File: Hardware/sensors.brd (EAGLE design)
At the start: 45.7 x 35.6 mm, 19 parts, among them IC1 74AC11D, IC2 REG1117

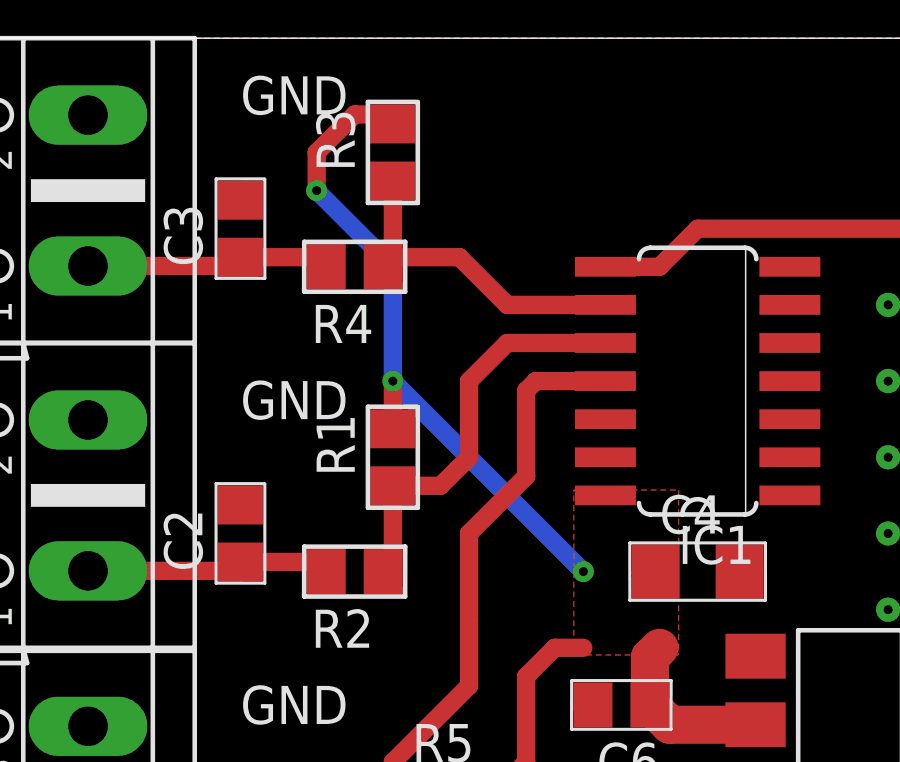
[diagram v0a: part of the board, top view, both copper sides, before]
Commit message: Fix some componenent manufacturer reference
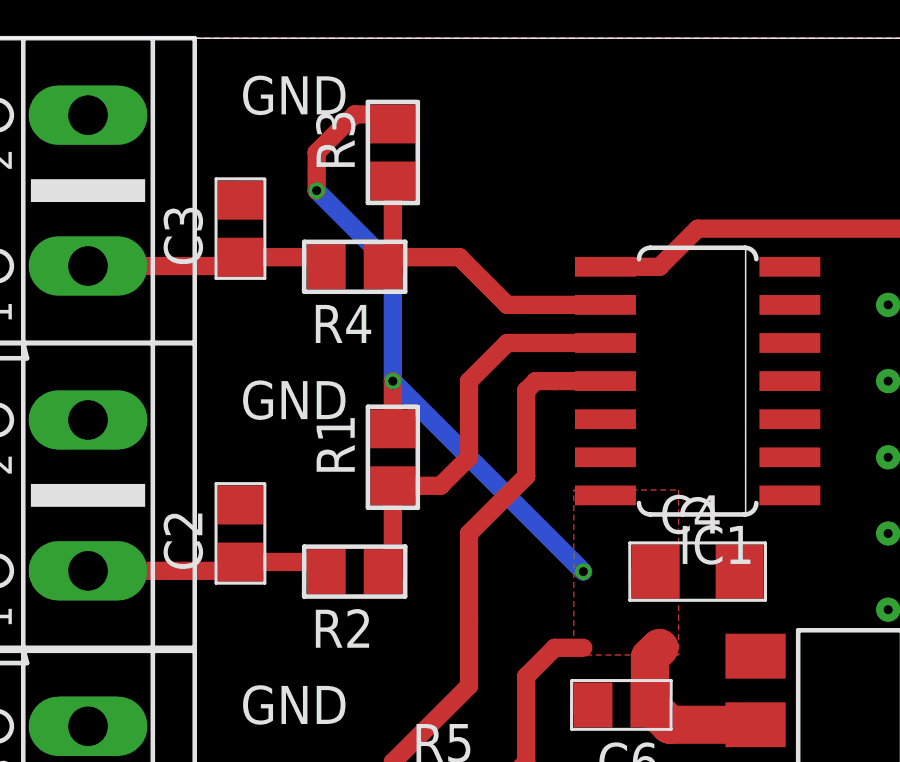
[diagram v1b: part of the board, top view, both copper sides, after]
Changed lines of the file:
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@@
 </class>
 </classes>
-<designrules name="default *">
-<description language="de">&lt;b&gt;EAGLE Design Rules&lt;/b&gt;
+<designrules name="jlcpcb2layer">
+<description language="en">&lt;b&gt;JLCPCB Design Rules by Jaap de Dood&lt;/b&gt;
 &lt;p&gt;
-Die Standard-Design-Rules sind so gewählt, dass sie für
-die meisten Anwendungen passen. Sollte ihre Platine
-besondere Anforderungen haben, treffen Sie die erforderlichen
-Einstellungen hier und speichern die Design Rules unter
-einem neuen Namen ab.</description>
-<description language="en">&lt;b&gt;EAGLE Design Rules&lt;/b&gt;
-&lt;p&gt;
-The default Design Rules have been set to cover
-a wide range of applications. Your particular design
-may have different requirements, so please make the
-necessary adjustments and save your customized
-design rules under a new name.</description>
+Please make sure your boards conform to these design rules.
+&lt;/p&gt;</description>
 <param name="layerSetup" value="(1*16)"/>
 <param name="mtCopper" value="0.035mm 0.035mm 0.035mm 0.035mm 0.035mm 0.035mm 0.035mm 0.035mm 0.035mm 0.035mm 0.035mm 0.035mm 0.035mm 0.035mm 0.035mm 0.035mm"/>
-<param name="mtIsolate" value="1.5mm 0.15mm 0.2mm 0.15mm 0.2mm 0.15mm 0.2mm 0.15mm 0.2mm 0.15mm 0.2mm 0.15mm 0.2mm 0.15mm 0.2mm"/>
-<param name="mdWireWire" value="8mil"/>
-<param name="mdWirePad" value="8mil"/>
-<param name="mdWireVia" value="8mil"/>
-<param name="mdPadPad" value="8mil"/>
-<param name="mdPadVia" value="8mil"/>
-<param name="mdViaVia" value="8mil"/>
-<param name="mdSmdPad" value="8mil"/>
-<param name="mdSmdVia" value="8mil"/>
-<param name="mdSmdSmd" value="8mil"/>
+<param name="mtIsolate" value="1.6mm 0.15mm 0.2mm 0.15mm 0.2mm 0.15mm 0.2mm 0.15mm 0.2mm 0.15mm 0.2mm 0.15mm 0.2mm 0.15mm 0.2mm"/>
+<param name="mdWireWire" value="5mil"/>
+<param name="mdWirePad" value="5mil"/>
+<param name="mdWireVia" value="5mil"/>
+<param name="mdPadPad" value="5mil"/>
+<param name="mdPadVia" value="5mil"/>
+<param name="mdViaVia" value="5mil"/>
+<param name="mdSmdPad" value="5mil"/>
+<param name="mdSmdVia" value="5mil"/>
+<param name="mdSmdSmd" value="5mil"/>
 <param name="mdViaViaSameLayer" value="8mil"/>
 <param name="mnLayersViaInSmd" value="2"/>
-<param name="mdCopperDimension" value="16mil"/>
-<param name="mdDrill" value="8mil"/>
+<param name="mdCopperDimension" value="8mil"/>
+<param name="mdDrill" value="0.5mm"/>
 <param name="mdSmdStop" value="0mil"/>
-<param name="msWidth" value="8mil"/>
-<param name="msDrill" value="8mil"/>
-<param name="msMicroVia" value="9.99mm"/>
+<param name="msWidth" value="5mil"/>
+<param name="msDrill" value="0.2mm"/>
+<param name="msMicroVia" value="0.2mm"/>
 <param name="msBlindViaRatio" value="0.5"/>
 <param name="rvPadTop" value="0.25"/>
@@
 <param name="rvMicroViaOuter" value="0.25"/>
 <param name="rvMicroViaInner" value="0.25"/>
-<param name="rlMinPadTop" value="10mil"/>
+<param name="rlMinPadTop" value="0.13mm"/>
 <param name="rlMaxPadTop" value="20mil"/>
-<param name="rlMinPadInner" value="10mil"/>
+<param name="rlMinPadInner" value="0.13mm"/>
 <param name="rlMaxPadInner" value="20mil"/>
-<param name="rlMinPadBottom" value="10mil"/>
+<param name="rlMinPadBottom" value="0.13mm"/>
 <param name="rlMaxPadBottom" value="20mil"/>
-<param name="rlMinViaOuter" value="8mil"/>
+<param name="rlMinViaOuter" value="0.13mm"/>
 <param name="rlMaxViaOuter" value="20mil"/>
-<param name="rlMinViaInner" value="8mil"/>
+<param name="rlMinViaInner" value="0.13mm"/>
 <param name="rlMaxViaInner" value="20mil"/>
-<param name="rlMinMicroViaOuter" value="4mil"/>
+<param name="rlMinMicroViaOuter" value="0.13mm"/>
 <param name="rlMaxMicroViaOuter" value="20mil"/>
-<param name="rlMinMicroViaInner" value="4mil"/>
+<param name="rlMinMicroViaInner" value="0.13mm"/>
 <param name="rlMaxMicroViaInner" value="20mil"/>
 <param name="psTop" value="-1"/>
@@
 <param name="mvStopFrame" value="1"/>
 <param name="mvCreamFrame" value="0"/>
-<param name="mlMinStopFrame" value="4mil"/>
-<param name="mlMaxStopFrame" value="4mil"/>
-<param name="mlMinCreamFrame" value="0mil"/>
+<param name="mlMinStopFrame" value="0.05mm"/>
+<param name="mlMaxStopFrame" value="2.5mil"/>
+<param name="mlMinCreamFrame" value="0.05mm"/>
 <param name="mlMaxCreamFrame" value="0mil"/>
-<param name="mlViaStopLimit" value="0mil"/>
+<param name="mlViaStopLimit" value="40mil"/>
 <param name="srRoundness" value="0"/>
 <param name="srMinRoundness" value="0mil"/>
